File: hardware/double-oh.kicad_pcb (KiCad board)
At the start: 2 copper layers, 81.6 x 14 mm, 54 parts, among them J1 USB_B_Micro, J10 Conn_01x01, J11 Conn_01x01, J12 Conn_01x01, J13 Conn_01x01, J2 Conn_01x01, J3 Conn_01x01, J4 Conn_01x01, J5 Conn_01x01, J6 Conn_01x01, J7 Conn_01x01, J8 Conn_01x01, J9 Conn_01x01, Q1 Q_DUAL_NPN_NPN_E1B1C2E2B2C1, Q2 Q_PMOS_GSD, Q3 Q_PMOS_GSD, U1 MCP73831-2-OT, U2 CP2104, U3 TPSM828x, U4 ESP32-U4WDH, U5 XC6120CxxxHR, U6 TPSM828x

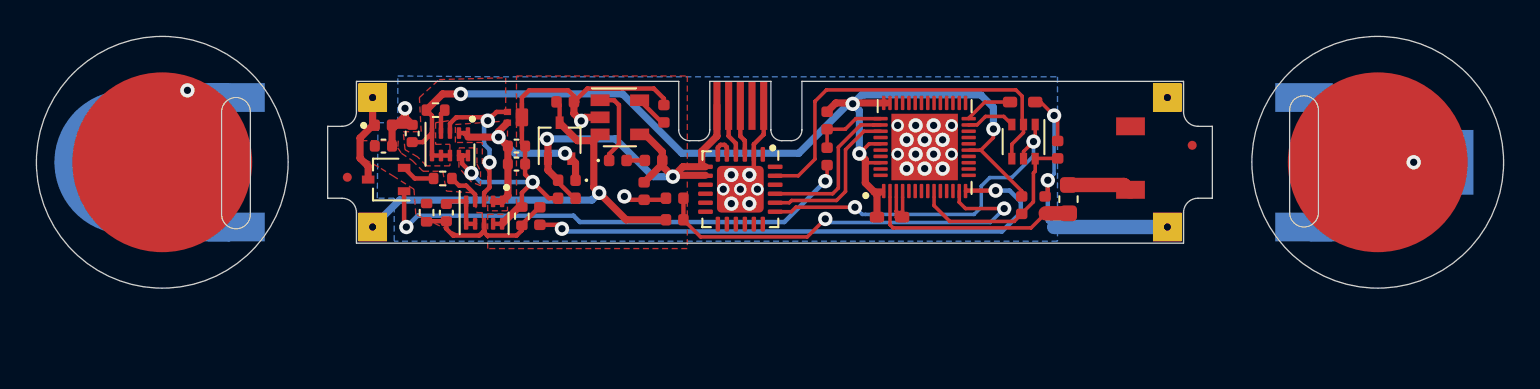
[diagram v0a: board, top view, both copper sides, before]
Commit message: To be continued
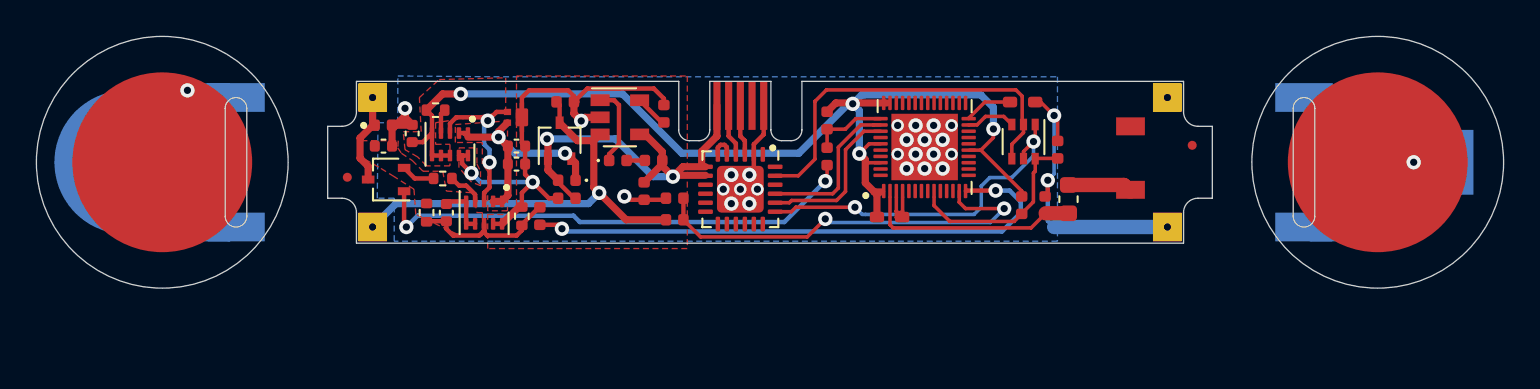
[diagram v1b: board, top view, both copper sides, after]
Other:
- outline, holes or cut-outs redrawn

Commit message: working on condensing the board
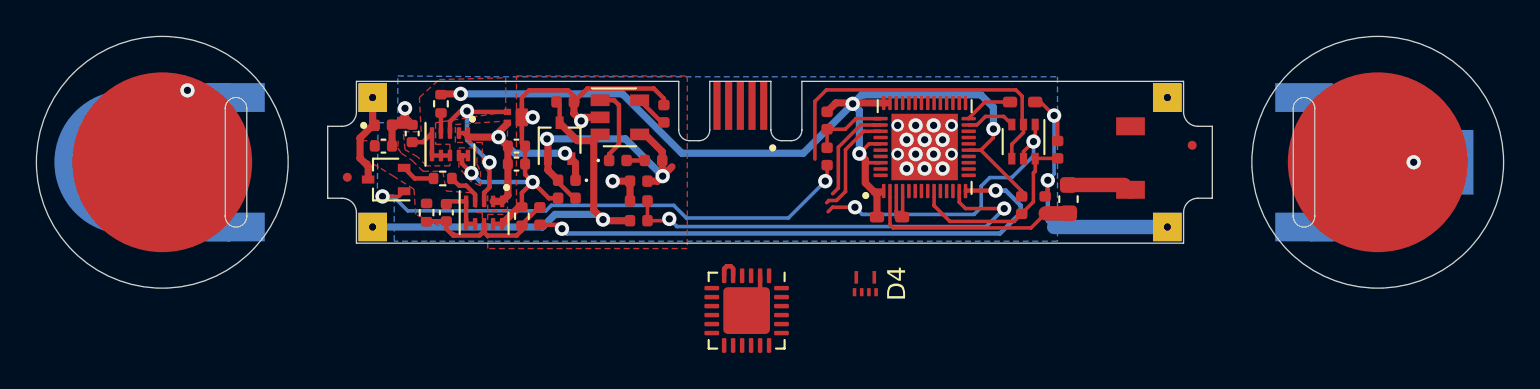
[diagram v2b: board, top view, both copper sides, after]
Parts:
- added D4: RCLAMP1624T, double-oh:SLP1710P4T, F.Cu at (128.3, 111.2)
- U3, U6: value TPSM828x -> TPSM8282x
- moved U2 6.76 mm to (121.7, 112.8)
- moved R3 2.01 mm to (115.7, 106.7)
- moved R1 2.00 mm to (115.7, 107.8)
- moved C1 0.63 mm to (115.7, 105.5), turned to 0 degrees
- moved R6 0.46 mm to (104.7, 101.2), turned to 270 degrees
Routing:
- net USB_VIN: track 24.5 -> 16.3 mm
- net RX_ESP: track 8.78 -> 5.58 mm
- net RTS: track 19.7 -> 16.7 mm
- net Net-(D4-Pad2): track 2.88 -> 0.00 mm
- net RX_USB: track 8.87 -> 6.01 mm
- net Net-(D4-Pad3): track 2.82 -> 0.00 mm
- net 0V: track 55.9 -> 53.2 mm, vias 28 -> 22
- net 3.3V: track 60.4 -> 57.7 mm
- net DTR: track 21.5 -> 18.9 mm
- net LIPO_V: track 24.8 -> 23.4 mm
- net ADC: track 23.6 -> 24.8 mm
- net Net-(Q2-Pad1): track 27.8 -> 28.7 mm
- net TPS_EN: track 8.97 -> 9.77 mm
